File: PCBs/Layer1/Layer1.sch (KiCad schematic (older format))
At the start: 46 parts, among them J1 Screw_Terminal_01x02, J2 Conn_01x12, T1 T60404-E4624-X501, U1 STPM_STPM10BTR, U2 level_shifter, U3 Micro_SD_Shield, U4 DOIT_ESP32_Devkit_v1-MCU_Modu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, Y1 4.194304 MHz

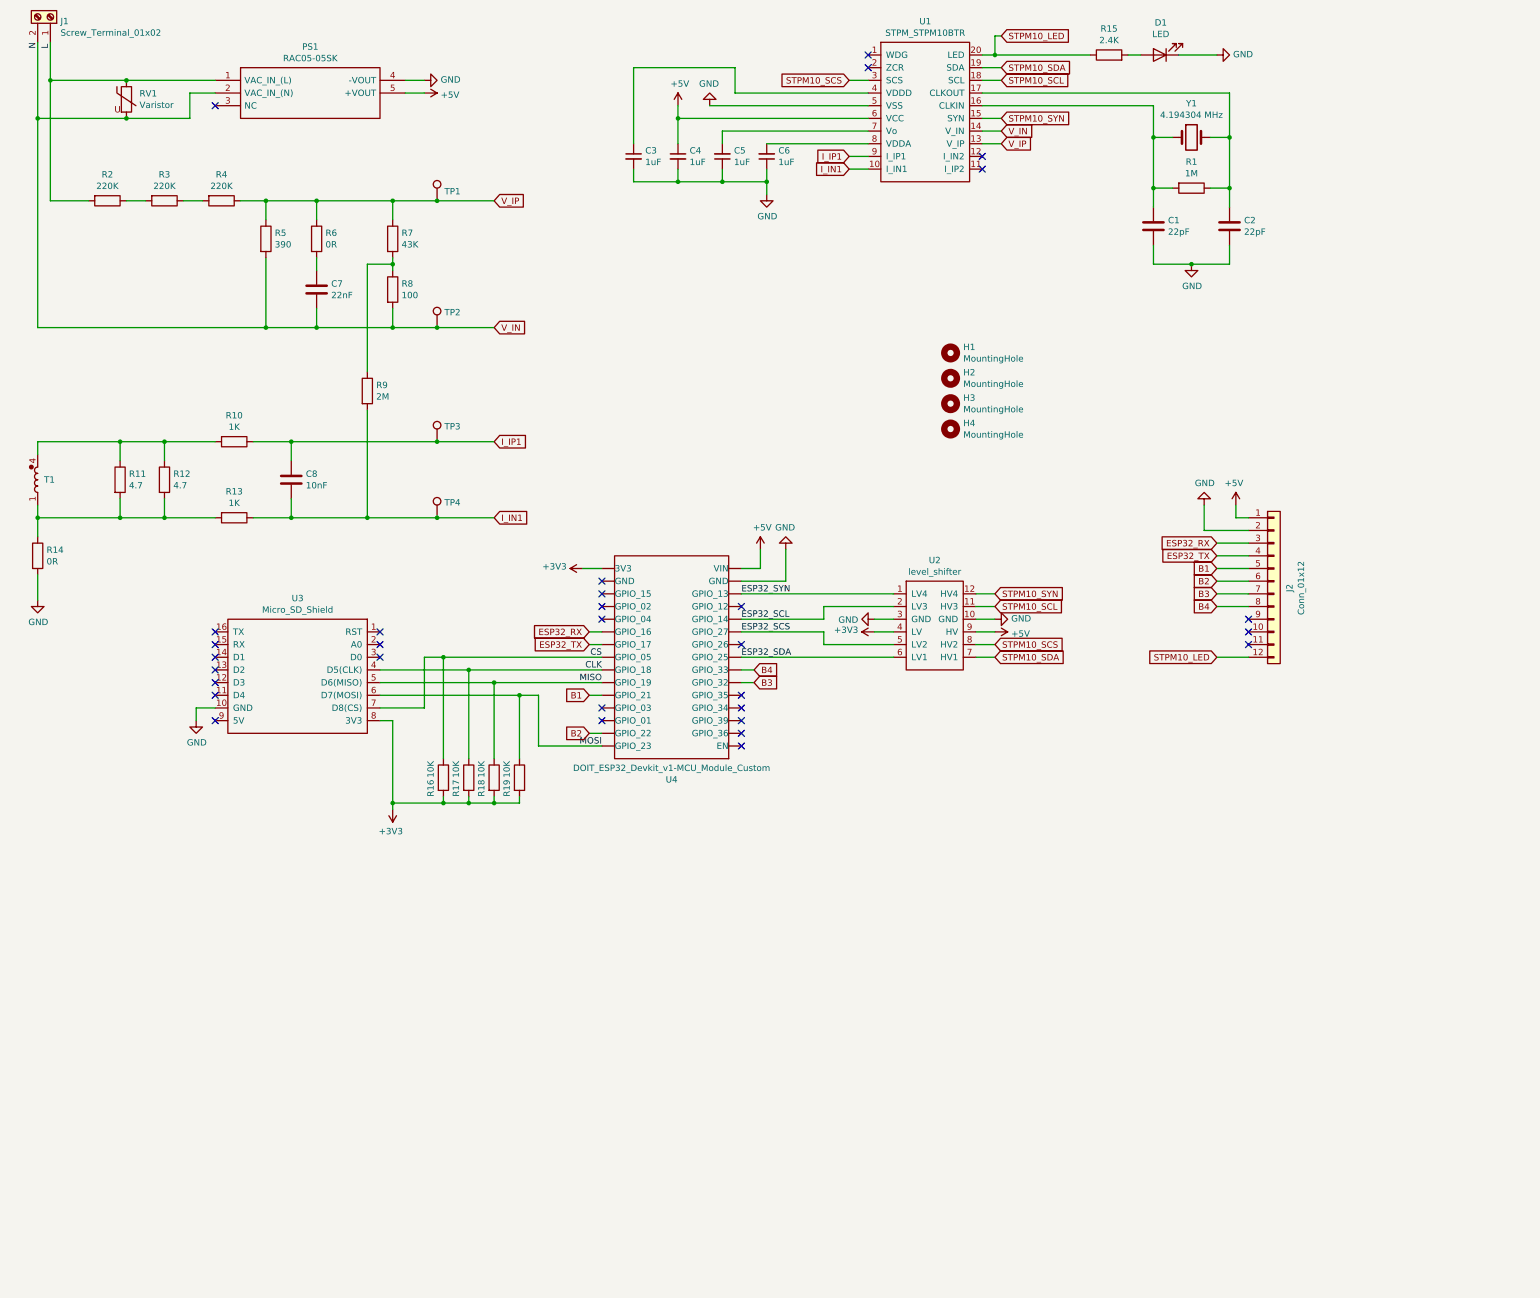
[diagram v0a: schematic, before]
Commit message: WIP: version 2
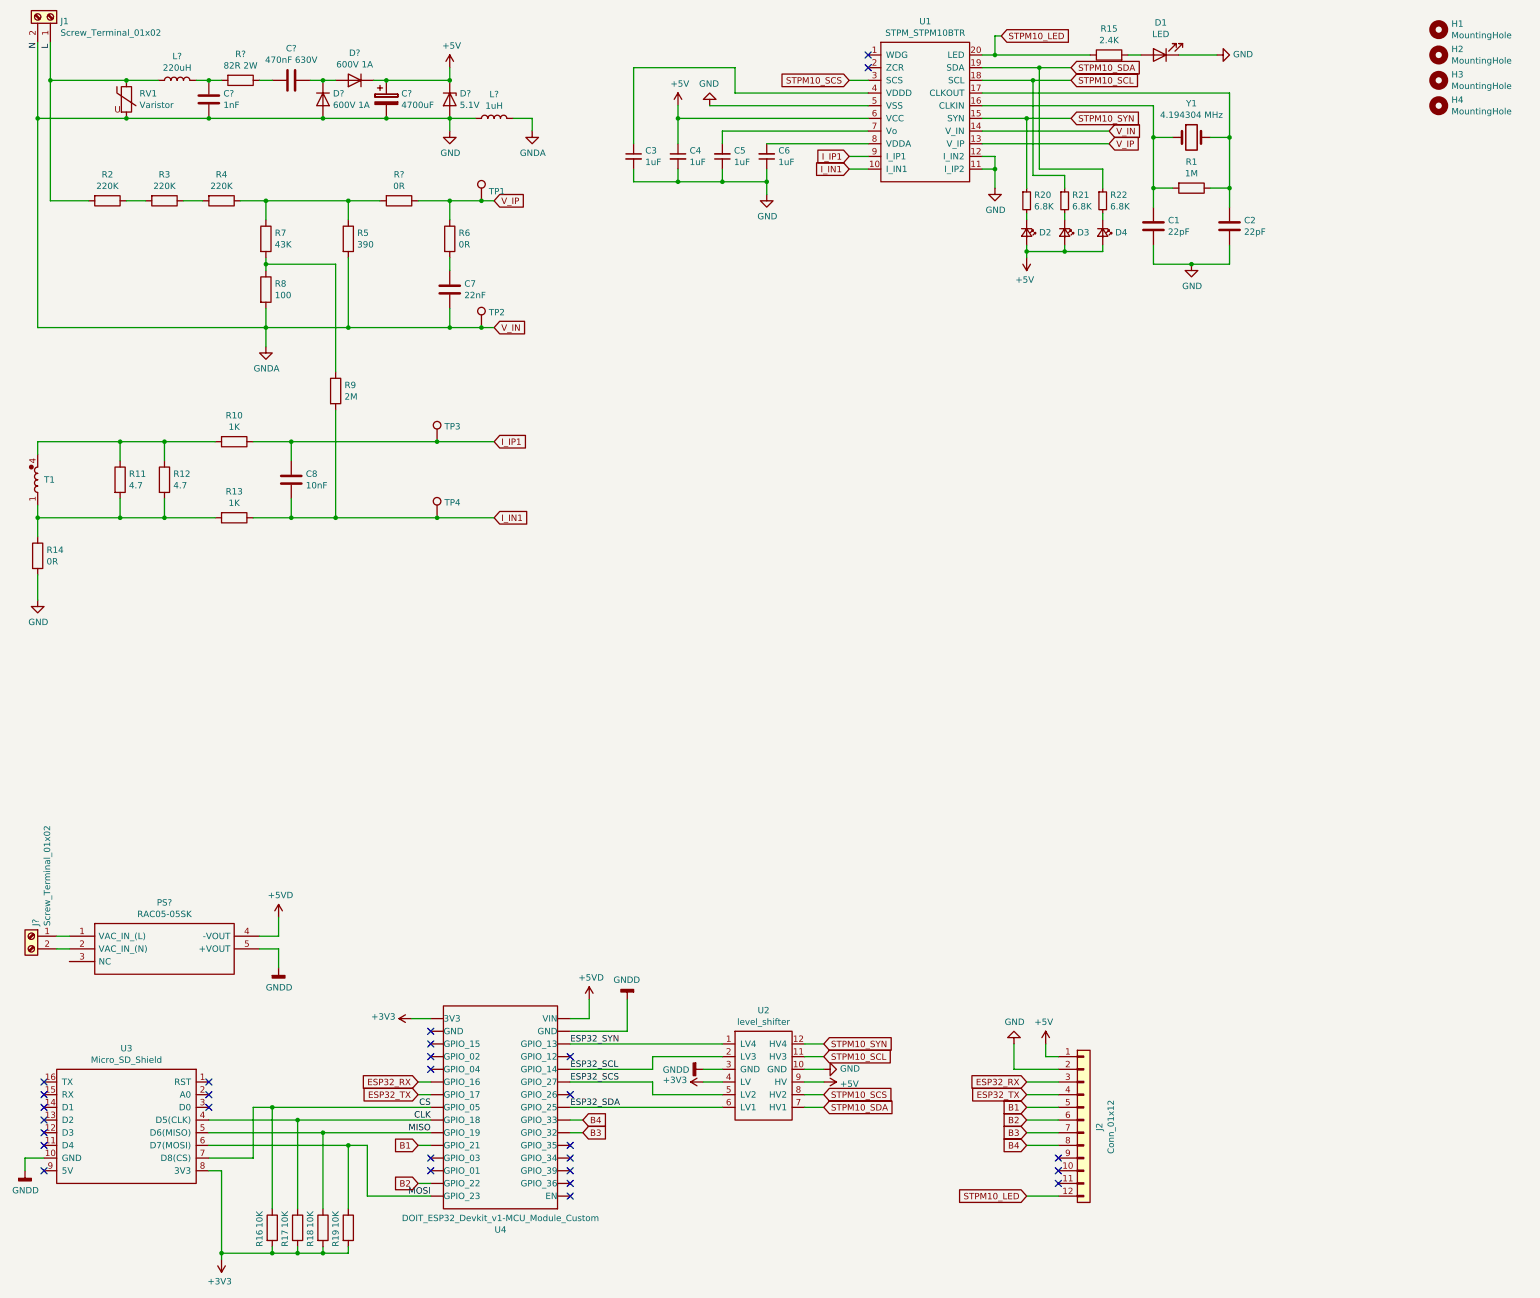
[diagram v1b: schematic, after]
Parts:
- removed PS1: RAC05-05SK, RAC05-05SK:RAC05-12SK, symbol RAC05-05SK:RAC05-05SK
- added C?: 1nF, symbol Device:C
- added C?: 470nF 630V, symbol Device:C
- added C?: 4700uF, symbol Device:CP
- added D2, D3, D4: LED_Small, LED_SMD:LED_0603_1608Metric_Pad1.05x0.95mm_HandSolder, symbol Device:LED_Small
- added D? (x2): 600V 1A, symbol Device:D
- added D?: 5.1V, symbol Device:D_Zener
- added J?: Screw_Terminal_01x02, TerminalBlock:TerminalBlock_bornier-2_P5.08mm, symbol Connector:Screw_Terminal_01x02
- added L?: 220uH, symbol Device:L
- added L?: 1uH, symbol Device:L
- added PS?: RAC05-05SK, RAC05-12SK, symbol RAC05-05SK:RAC05-05SK
- added R20, R21, R22: 6.8K, Resistor_SMD:R_0603_1608Metric_Pad1.05x0.95mm_HandSolder, symbol Device:R_Small
- added R?: 82R 2W, symbol Device:R
- added R?: 0R, symbol Device:R
- C3, C4, C5, C6: footprint Capacitor_SMD:C_1206_3216Metric_Pad1.42x1.75mm_HandSolder -> Capacitor_SMD:C_0603_1608Metric_Pad1.05x0.95mm_HandSolder
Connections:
- net V_IN is gone; now on net GND: C7.2, J1.2 (Pin_2), R5.2, R8.2, RV1.2, TP2.1, U1.14 (V_IN)
- net +5V: now also C?.1, D2.2 (A), D3.2 (A), D4.2 (A), D?.1 (K), D?.1 (K); no longer U4.15 (VIN)
- net GND: now also U1.11 (I_IP2), U1.12 (I_IN2), C?.2, C?.2, D?.2 (A), D?.2 (A), L?.1, L?.2; no longer U2.3 (GND), U3.10 (GND), U4.14 (GND)
- net L: now also L?.1
- net STPM10_SCL: now also R21.1
- net STPM10_SDA: now also R22.1
- net STPM10_SYN: now also R20.1
- net V_IP: now also R?.1; no longer R4.1, R5.1, R7.1
- new net: R4.1, R5.1, R7.1, R?.2
- new net: D2.1 (K), R20.2
- new net: C?.1, L?.2, R?.2
- new net: C?.2, R?.1
- new net: C?.1, D?.1 (K), D?.2 (A)
- new net: D3.1 (K), R21.2
- new net: D4.1 (K), R22.2
- new net: J?.1 (Pin_1), PS?.1 (VAC_IN_(L))
- new net: J?.2 (Pin_2), PS?.2 (VAC_IN_(N))
- new net +5VD: PS?.4 (-VOUT), U4.15 (VIN)
- new net GNDD: PS?.5 (+VOUT), U2.3 (GND), U3.10 (GND), U4.14 (GND)
- no-connect marks 31 -> 28
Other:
- moved on the sheet: C7, H1, H2, H3, H4, J2, R16, R17, R18, R19, R5, R6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
